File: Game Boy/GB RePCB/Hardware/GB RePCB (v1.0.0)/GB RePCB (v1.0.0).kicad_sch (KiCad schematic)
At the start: 0 parts

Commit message: GB RePCB LH5264 Schematic
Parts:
- added U1: LH5264, Package_SO:SOP-28_8.4x18.16mm_P1.27mm, symbol RetroSix Library:LH5264
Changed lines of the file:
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@@
 	(generator_version "9.0")
 	(paper "A4")
+	(symbol
+		(lib_id "RetroSix Library:LH5264")
+		(at 133.35 127 0)
+		(unit 1)
+		(exclude_from_sim no)
+		(in_bom yes)
+		(on_board yes)
+		(dnp no)
+		(property "Reference" "U1"
+			(at 147.32 76.2 0)
+			(effects
+				(font
+					(size 1.27 1.27)
+				)
+			)
+		)
+		(property "Value" "LH5264"
+			(at 147.32 78.74 0)
+			(effects
+				(font
+					(size 1.27 1.27)
+				)
+			)
+		)
+		(property "Footprint" "Package_SO:SOP-28_8.4x18.16mm_P1.27mm"
+			(at 143.256 138.43 0)
+			(effects
+				(font
+					(size 1.27 1.27)
+				)
+				(hide yes)
+			)
+		)
+		(property "Datasheet" "https://www.alliancememory.com/wp-content/uploads/Alliance-Memory_64K_AS6C6264v2.0July2017.pdf"
+			(at 142.494 136.144 0)
+			(effects
+				(font
+					(size 1.27 1.27)
+				)
+				(hide yes)
+			)
+		)
+		(property "Description" "8K X 8 BIT LOW POWER CMOS SRAM. Alternative Part Number AS6C6264"
+			(at 141.732 134.112 0)
+			(effects
+				(font
+					(size 1.27 1.27)
+				)
+				(hide yes)
+			)
+		)
+		(property "Manufacturer" "Sharp"
+			(at 143.256 132.08 0)
+			(effects
+				(font
+					(size 1.27 1.27)
+				)
+				(hide yes)
+			)
+		)
+		(pin "10"
+		)
+		(pin "6"
+		)
+		(pin "28"
+		)
+		(pin "9"
+		)
+		(pin "8"
+		)
+		(pin "7"
+		)
+		(pin "5"
+		)
+		(pin "4"
+		)
+		(pin "3"
+		)
+		(pin "19"
+		)
+		(pin "1"
+		)
+		(pin "12"
+		)
+		(pin "13"
+		)
+		(pin "15"
+		)
+		(pin "16"
+		)
+		(pin "17"
+		)
+		(pin "18"
+		)
+		(pin "25"
+		)
+		(pin "24"
+		)
+		(pin "21"
+		)
+		(pin "23"
+		)
+		(pin "2"
+		)
+		(pin "14"
+		)
+		(pin "27"
+		)
+		(pin "22"
+		)
+		(pin "20"
+		)
+		(pin "26"
+		)
+		(pin "11"
+		)
+		(instances
+			(project ""
+				(path "/9333ae1f-effc-4f90-9e00-d8a86e0893b0"
+					(reference "U1")
+					(unit 1)
+				)
+			)
+		)
+	)
 	(sheet_instances
 		(path "/"

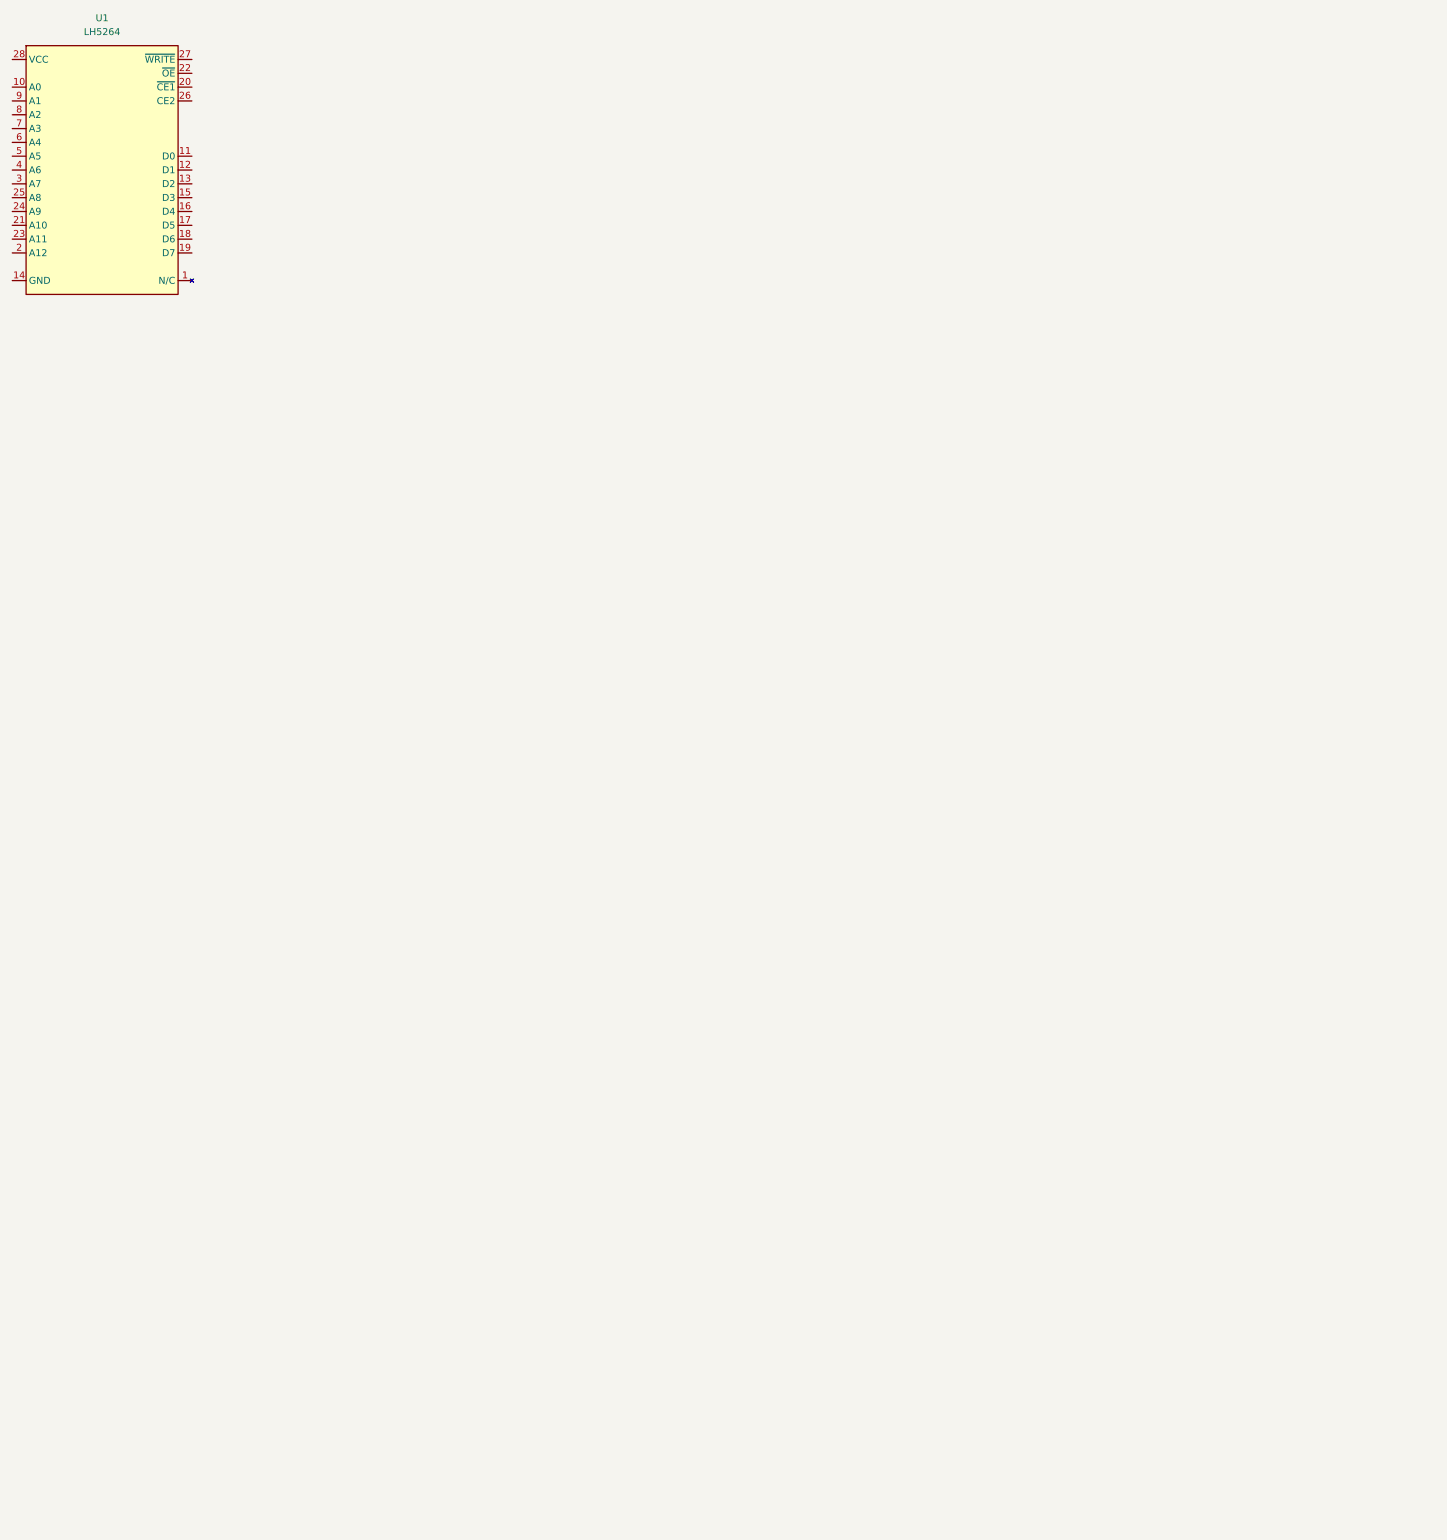
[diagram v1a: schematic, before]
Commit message: GB RePCB CPU schematic
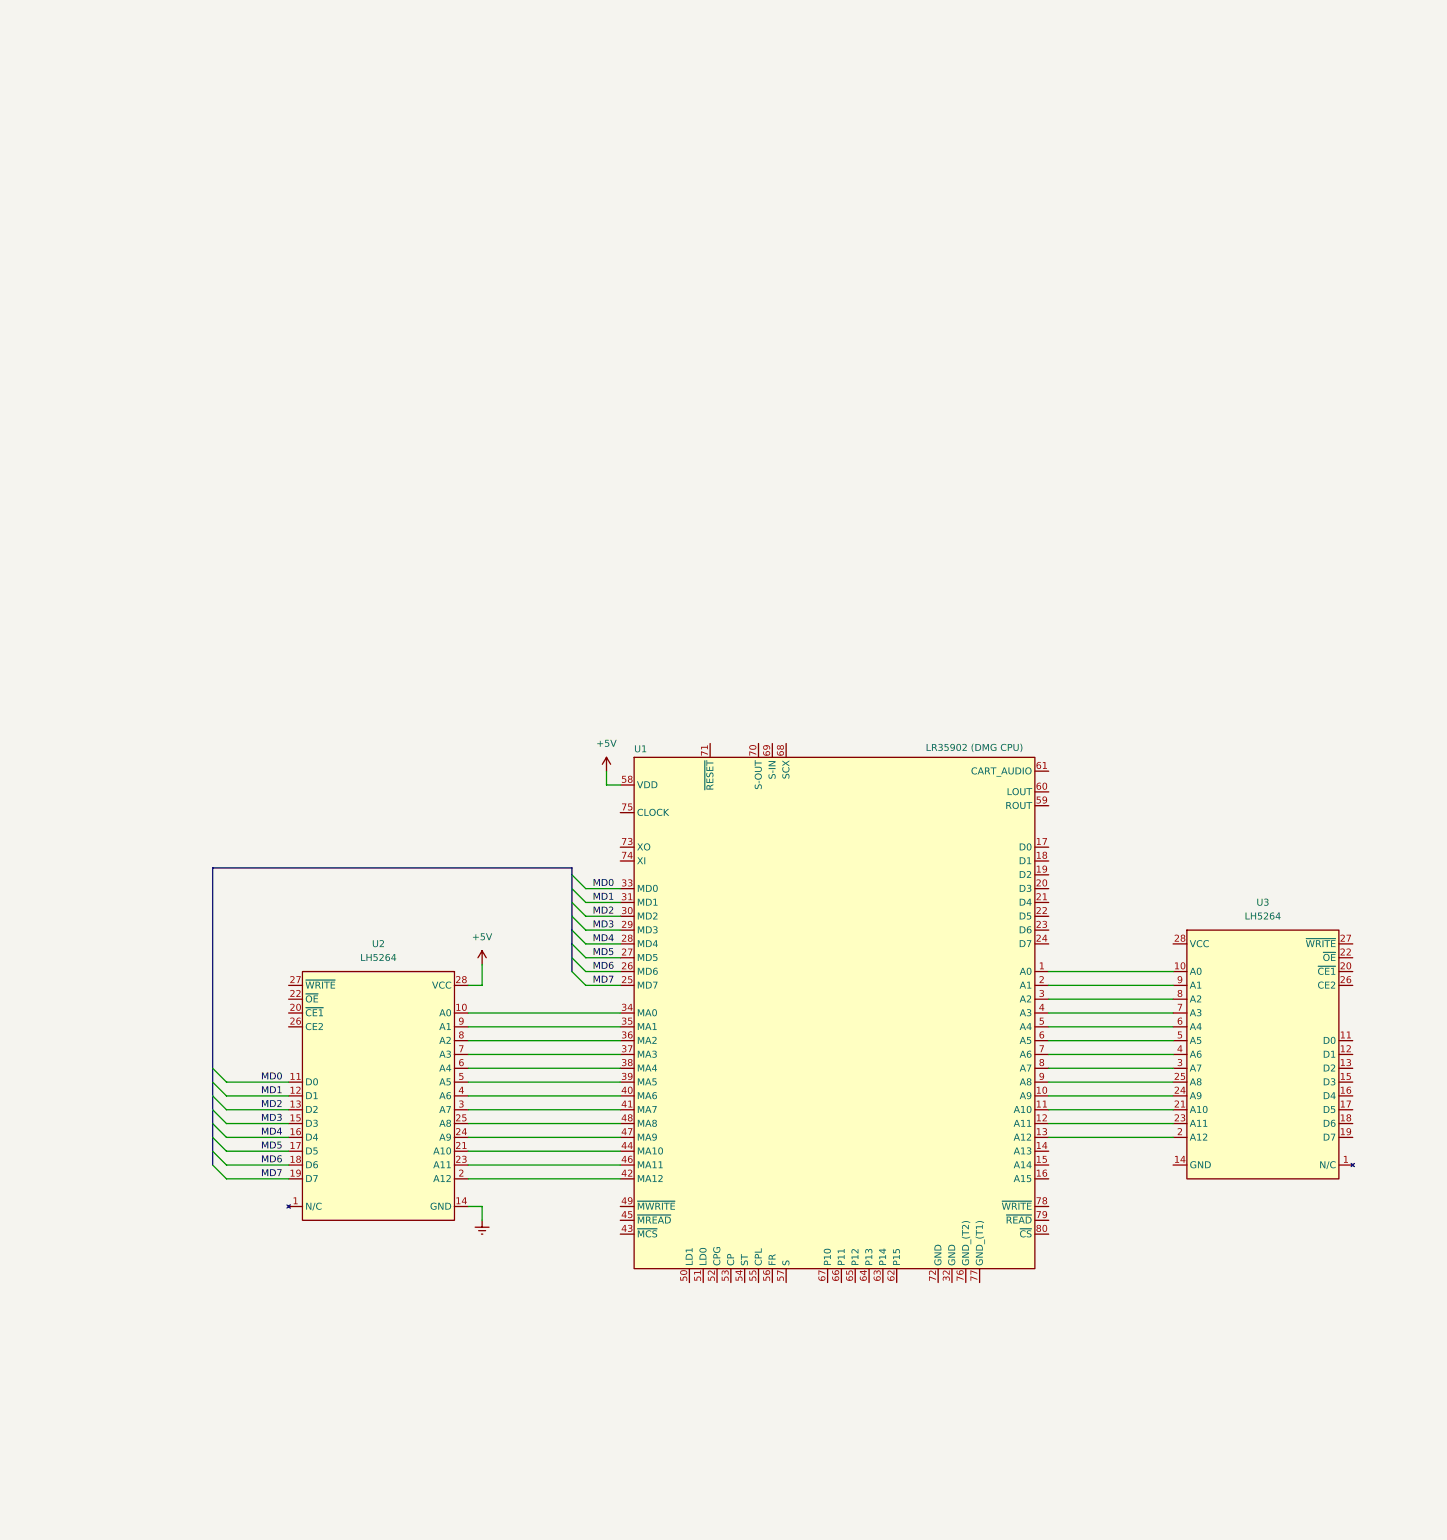
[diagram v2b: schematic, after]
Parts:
- added U1: LR35902 (DMG CPU), symbol RetroSix Library:LR35902_(DMG_CPU)
- added U2: LH5264, Package_SO:SOP-28_8.4x18.16mm_P1.27mm, symbol RetroSix Library:LH5264
- renumbered U1 to U3
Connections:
- net at U3.10 (A0): now also U1.1 (A0)
- net at U3.2 (A12): now also U1.13 (A12)
- net at U3.21 (A10): now also U1.11 (A10)
- net at U3.23 (A11): now also U1.12 (A11)
- net at U3.24 (A9): now also U1.10 (A9)
- net at U3.25 (A8): now also U1.9 (A8)
- net at U3.3 (A7): now also U1.8 (A7)
- net at U3.4 (A6): now also U1.7 (A6)
- net at U3.5 (A5): now also U1.6 (A5)
- net at U3.6 (A4): now also U1.5 (A4)
- net at U3.7 (A3): now also U1.4 (A3)
- net at U3.8 (A2): now also U1.3 (A2)
- net at U3.9 (A1): now also U1.2 (A1)
- new net: U1.34 (MA0), U2.10 (A0)
- new net: U1.42 (MA12), U2.2 (A12)
- new net: U1.44 (MA10), U2.21 (A10)
- new net: U1.46 (MA11), U2.23 (A11)
- new net: U1.47 (MA9), U2.24 (A9)
- new net: U1.48 (MA8), U2.25 (A8)
- new net: U1.41 (MA7), U2.3 (A7)
- new net: U1.40 (MA6), U2.4 (A6)
- new net: U1.39 (MA5), U2.5 (A5)
- new net: U1.38 (MA4), U2.6 (A4)
- new net: U1.37 (MA3), U2.7 (A3)
- new net: U1.36 (MA2), U2.8 (A2)
- new net: U1.35 (MA1), U2.9 (A1)
- new net +5V: U1.58 (VDD), U2.28 (VCC)
- new net GNDREF: U2.14 (GND)
- new net MD0: U1.33 (MD0), U2.11 (D0)
- new net MD1: U1.31 (MD1), U2.12 (D1)
- new net MD2: U1.30 (MD2), U2.13 (D2)
- new net MD3: U1.29 (MD3), U2.15 (D3)
- new net MD4: U1.28 (MD4), U2.16 (D4)
- new net MD5: U1.27 (MD5), U2.17 (D5)
- new net MD6: U1.26 (MD6), U2.18 (D6)
- new net MD7: U1.25 (MD7), U2.19 (D7)
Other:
- moved on the sheet: U3

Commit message: GBO RePCB EXT Port
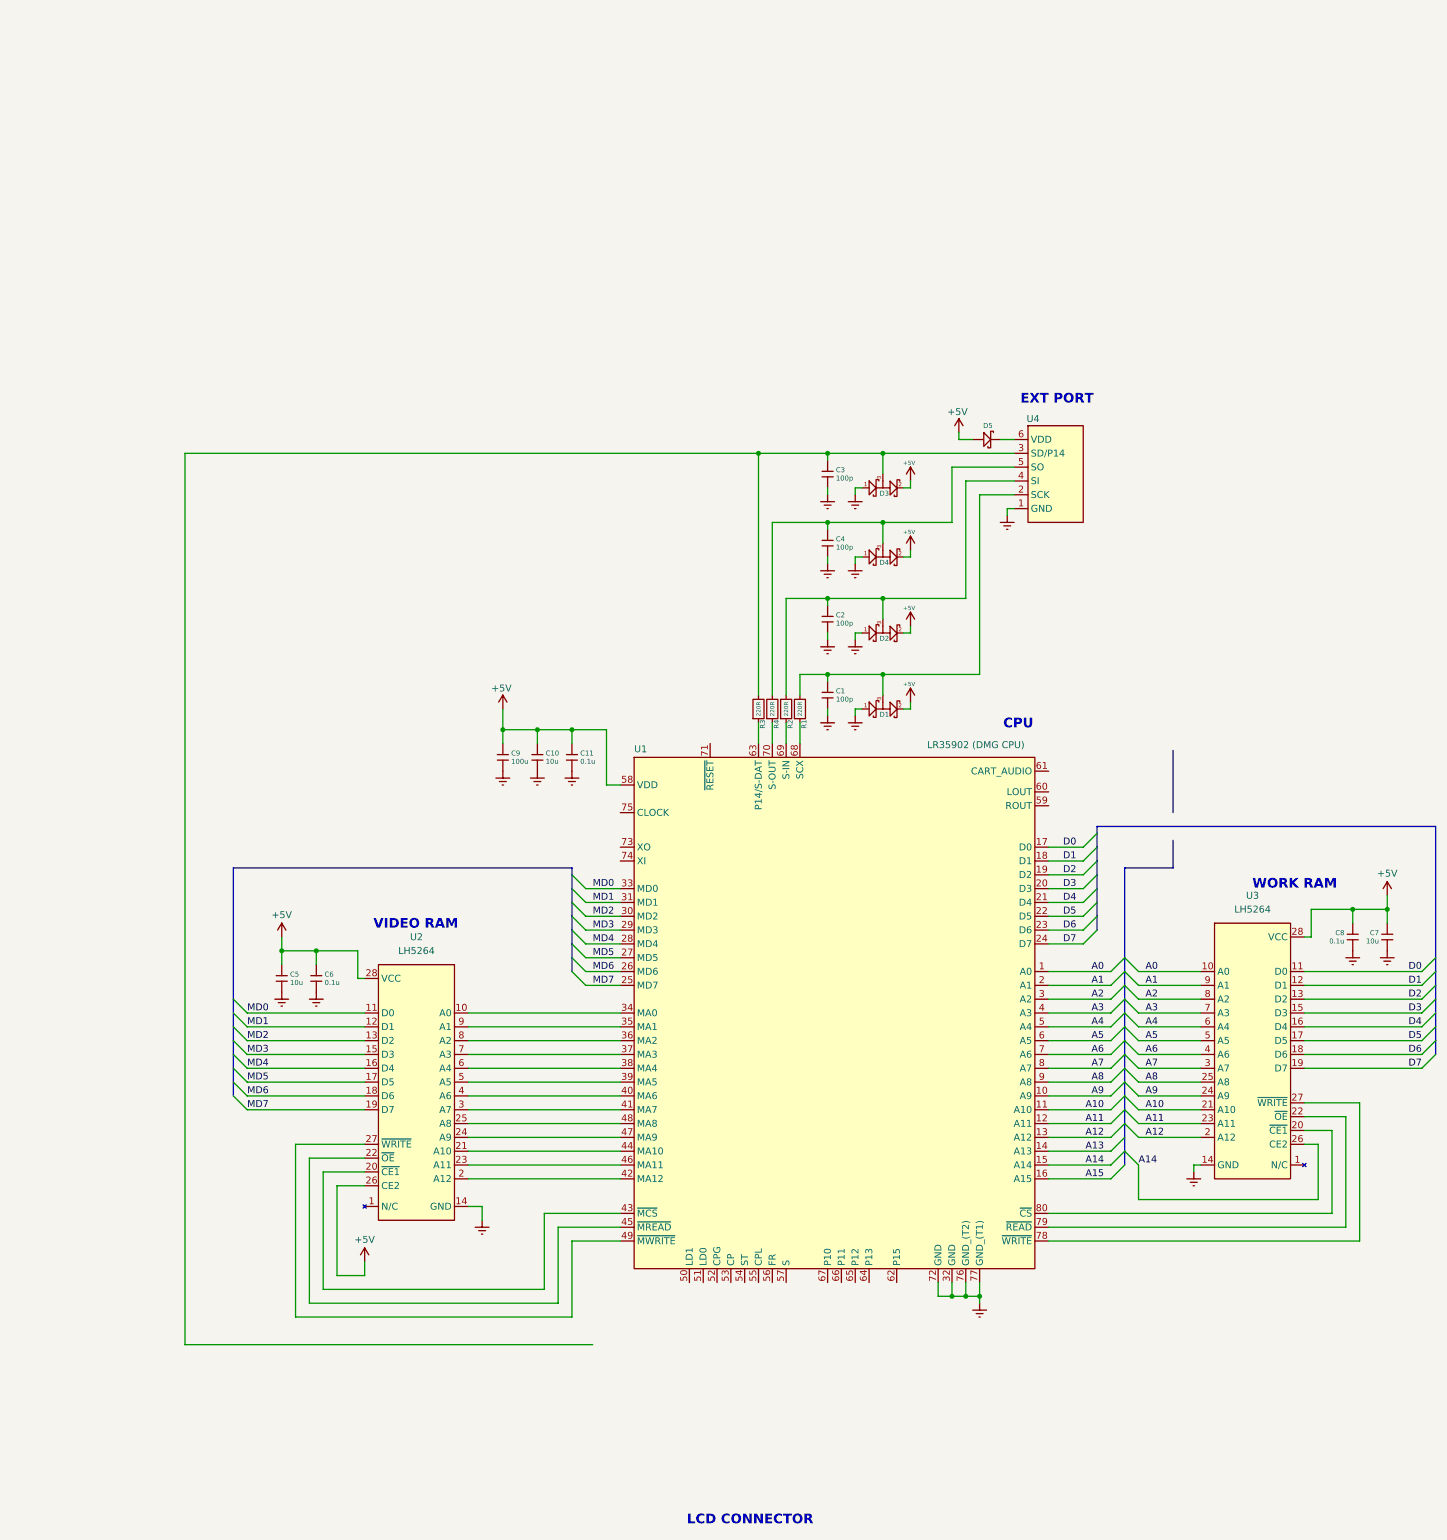
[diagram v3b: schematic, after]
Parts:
- removed U1: LR35902 (DMG CPU), symbol RetroSix Library:LR35902_(DMG_CPU)
- removed U2, U3: LH5264, Package_SO:SOP-28_8.4x18.16mm_P1.27mm, symbol RetroSix Library:LH5264
- added C1, C2, C3, C4: 100p, C0402, symbol Capacitors:CAP_0402
- added C10, C5, C7: 10u, C0402, symbol Capacitors:CAP_0402
- added C11, C6, C8: 0.1u, C0402, symbol Capacitors:CAP_0402
- added C9: 100u, C0402, symbol Capacitors:CAP_0402
- added D1, D2, D3, D4: BAT54S-7-F, Footprints:SOT23, symbol Diodes:BAT54S-7-F
- added D5: *, DO-214AC, symbol Diodes:SS14
- added R1, R2, R3, R4: 220R, R0402, symbol Resistors:RES_0402
- added U1: LR35902 (DMG CPU), symbol RetroSix Shared:LR35902_(DMG_CPU)
- added U2, U3: LH5264, Package_SO:SOP-28_8.4x18.16mm_P1.27mm, symbol RetroSix Shared:LH5264
- added U4: (no value), symbol RetroSix Shared:GBO-EXT-PORT
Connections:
- net +5V: now also C10.2, C11.2, C5.2, C6.2, C7.2, C8.2, C9.2, D1.2, D2.2, D3.2, D4.2, D5.A, U1.58 (VDD), U2.26 (CE2), U2.28 (VCC), U3.28 (VCC)
- net GNDREF: now also C1.1, C10.1, C11.1, C2.1, C3.1, C4.1, C5.1, C6.1, C7.1, C8.1, C9.1, D1.1, D2.1, D3.1, D4.1, U1.32 (GND), U1.72 (GND), U1.76 (GND_(T2)), U1.77 (GND_(T1)), U2.14 (GND), U3.14 (GND), U4.1 (GND)
- net MD0: now also U1.33 (MD0), U2.11 (D0)
- net MD1: now also U1.31 (MD1), U2.12 (D1)
- net MD2: now also U1.30 (MD2), U2.13 (D2)
- net MD3: now also U1.29 (MD3), U2.15 (D3)
- net MD4: now also U1.28 (MD4), U2.16 (D4)
- net MD5: now also U1.27 (MD5), U2.17 (D5)
- net MD6: now also U1.26 (MD6), U2.18 (D6)
- net MD7: now also U1.25 (MD7), U2.19 (D7)
- new net: R1.1, U1.68 (SCX)
- new net: C1.2, D1.3, R1.2, U4.2 (SCK)
- new net: U1.80 (~{CS}), U3.20 (~{CE1})
- new net: U1.79 (~{READ}), U3.22 (~{OE})
- new net: U1.78 (~{WRITE}), U3.27 (~{WRITE})
- new net: R4.1, U1.70 (S-OUT)
- new net: C4.2, D4.3, R4.2, U4.5 (SO)
- new net: U1.34 (MA0), U2.10 (A0)
- new net: U1.42 (MA12), U2.2 (A12)
- new net: U1.43 (~{MCS}), U2.20 (~{CE1})
- new net: U1.44 (MA10), U2.21 (A10)
- new net: U1.45 (~{MREAD}), U2.22 (~{OE})
- new net: U1.46 (MA11), U2.23 (A11)
- new net: U1.47 (MA9), U2.24 (A9)
- new net: U1.48 (MA8), U2.25 (A8)
- new net: U1.49 (~{MWRITE}), U2.27 (~{WRITE})
- new net: U1.41 (MA7), U2.3 (A7)
- new net: U1.40 (MA6), U2.4 (A6)
- new net: U1.39 (MA5), U2.5 (A5)
- new net: U1.38 (MA4), U2.6 (A4)
- new net: U1.37 (MA3), U2.7 (A3)
- new net: U1.36 (MA2), U2.8 (A2)
- new net: U1.35 (MA1), U2.9 (A1)
- new net: R3.1, U1.63 (P14/S-DAT)
- new net: C3.2, D3.3, R3.2, U4.3 (SD/P14)
- new net: R2.1, U1.69 (S-IN)
- new net: D5.C, U4.6 (VDD)
- new net: C2.2, D2.3, R2.2, U4.4 (SI)
- new net A0: U1.1 (A0), U3.10 (A0)
- new net A1: U1.2 (A1), U3.9 (A1)
- new net A10: U1.11 (A10), U3.21 (A10)
- new net A11: U1.12 (A11), U3.23 (A11)
- new net A12: U1.13 (A12), U3.2 (A12)
- new net A13: U1.14 (A13)
- new net A14: U1.15 (A14), U3.26 (CE2)
- new net A15: U1.16 (A15)
- new net A2: U1.3 (A2), U3.8 (A2)
- new net A3: U1.4 (A3), U3.7 (A3)
- new net A4: U1.5 (A4), U3.6 (A4)
- new net A5: U1.6 (A5), U3.5 (A5)
- new net A6: U1.7 (A6), U3.4 (A6)
- new net A7: U1.8 (A7), U3.3 (A7)
- new net A8: U1.9 (A8), U3.25 (A8)
- new net A9: U1.10 (A9), U3.24 (A9)
- new net D0: U1.17 (D0), U3.11 (D0)
- new net D1: U1.18 (D1), U3.12 (D1)
- new net D2: U1.19 (D2), U3.13 (D2)
- new net D3: U1.20 (D3), U3.15 (D3)
- new net D4: U1.21 (D4), U3.16 (D4)
- new net D5: U1.22 (D5), U3.17 (D5)
- new net D6: U1.23 (D6), U3.18 (D6)
- new net D7: U1.24 (D7), U3.19 (D7)
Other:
- note added: "CPU"
- note added: "EXT PORT"
- note added: "LCD CONNECTOR"
- note added: "VIDEO RAM"
- note added: "WORK RAM"
